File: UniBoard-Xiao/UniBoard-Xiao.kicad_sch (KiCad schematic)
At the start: 40 parts, among them J1 tirette, J10 I2C Extension, J11 LIDAR, J12 5vp, J13 5vp, J14 5vp, J15 ultrasonic sensor, J3 BAU, J4 oled I2C, J5 STEPPER D, J6 STEPPER G, J7 I2C Extension, J8 con BAT, J9 I2C Extension, SW1 SW_DIP_x02, SW2 SW_DIP_x02, U1 XIAO-ESP32-S3-DIP, U2 TMC2209_SILENTSTEPSTICK, U3 TMC2209_SILENTSTEPSTICK, U4 TSR1-2433E, U5 TSR2-2450N, U6 TSR1-2450E

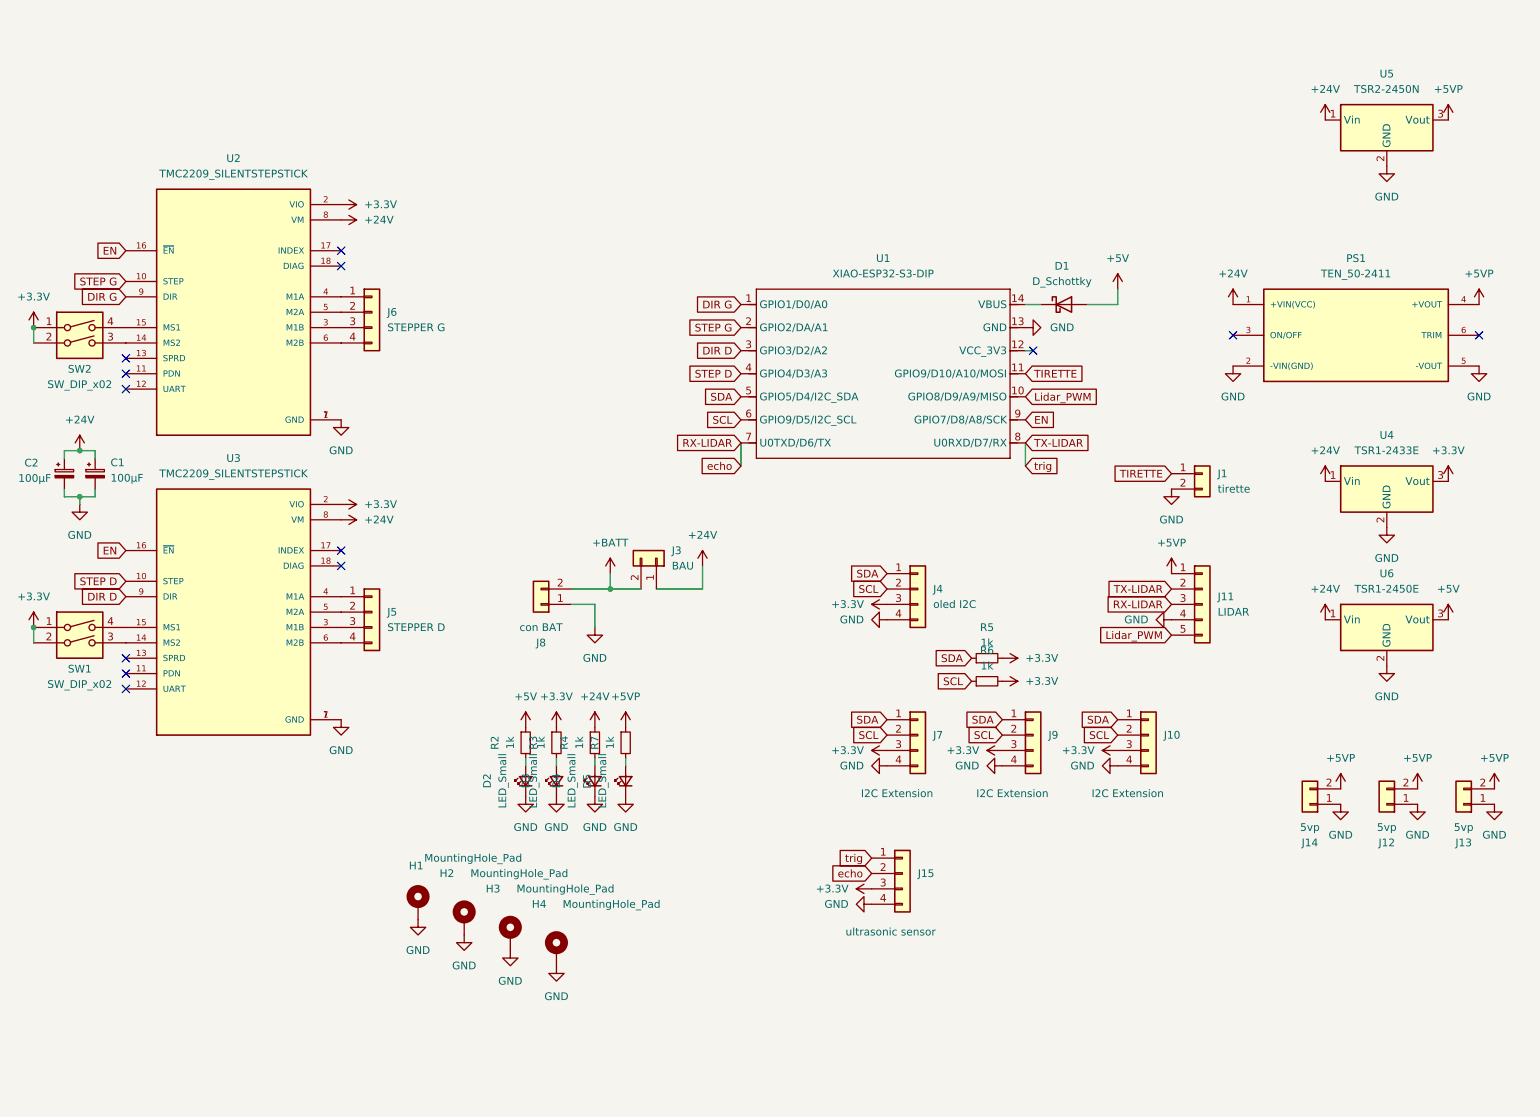
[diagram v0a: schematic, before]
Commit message: Refactor Schematic
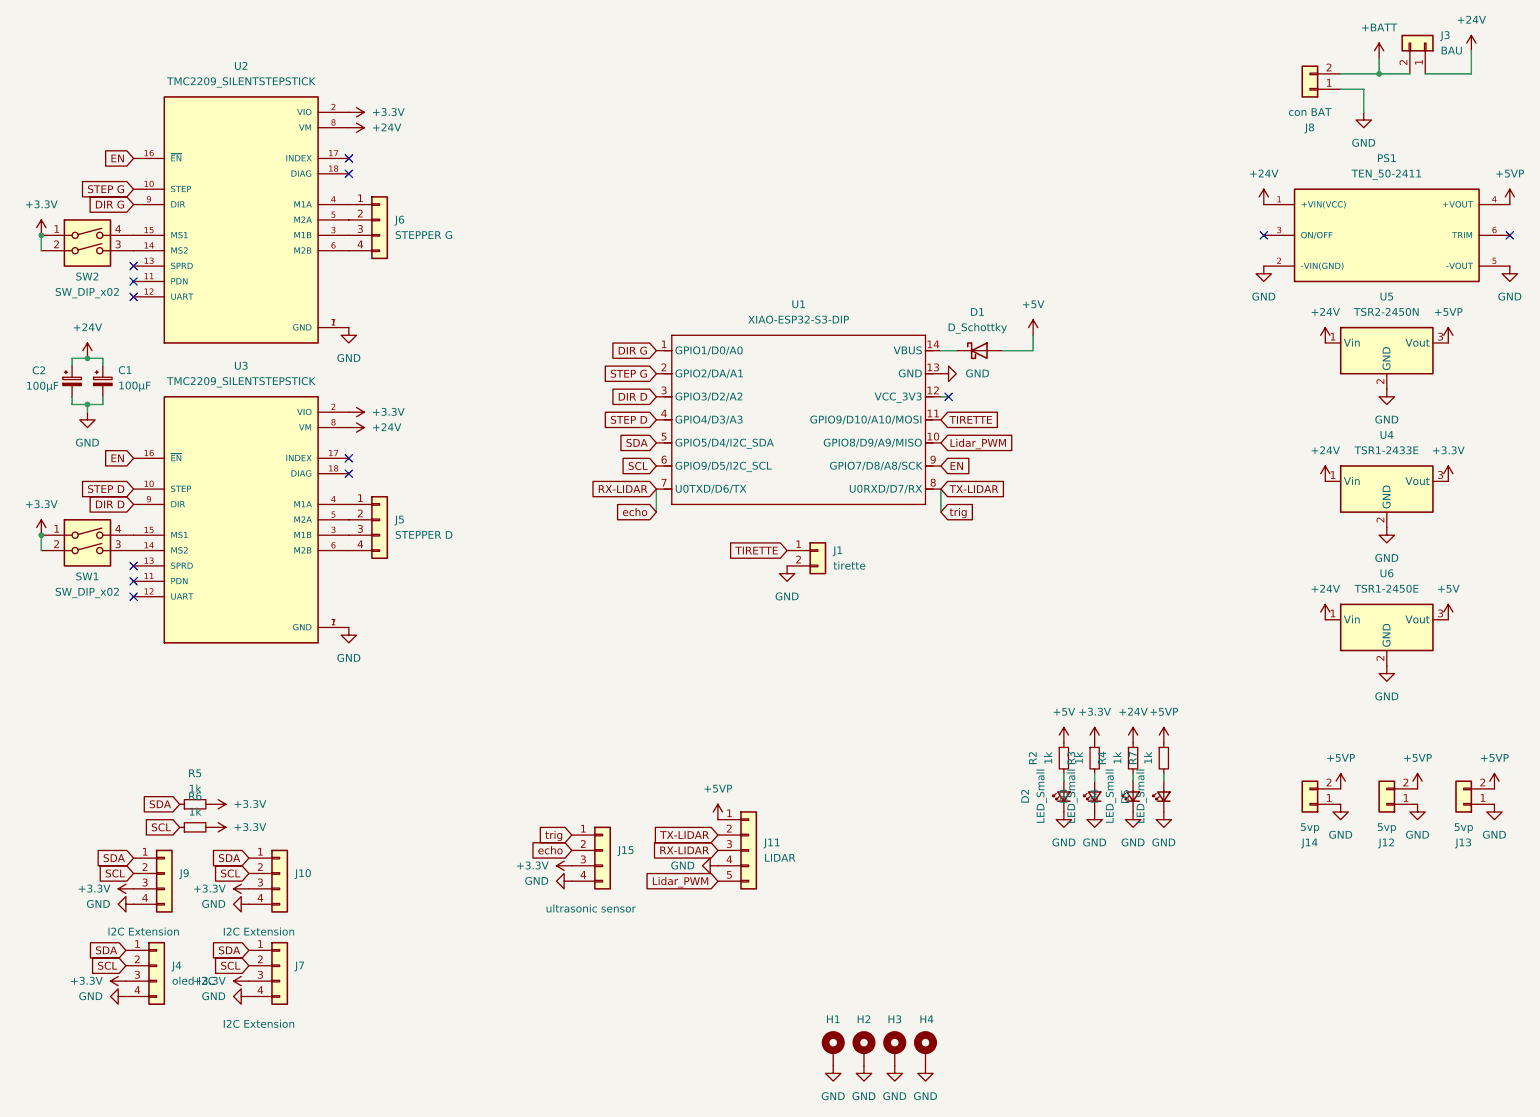
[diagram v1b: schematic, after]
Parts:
- H1, H2, H3, H4: now in the parts list
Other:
- moved on the sheet: C1, C2, D1, D2, D3, D4, D5, H1, H2, H3, H4, J1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
